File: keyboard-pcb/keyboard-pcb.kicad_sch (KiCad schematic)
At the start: 131 parts, among them SW1 RotaryEncoder_Switch, U1 Pico

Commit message: added footprints to pcb editor
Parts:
- U1: footprint RPi_Pico:RPi_Pico_SMD_TH -> MCU_RaspberryPi_and_Boards:RPi_Pico_SMD_TH
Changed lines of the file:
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@@
     (property "Reference" "U1" (id 0) (at 76.2 36.83 0))
     (property "Value" "Pico" (id 1) (at 76.2 39.37 0))
-    (property "Footprint" "RPi_Pico:RPi_Pico_SMD_TH" (id 2) (at 76.2 68.58 90)
+    (property "Footprint" "MCU_RaspberryPi_and_Boards:RPi_Pico_SMD_TH" (id 2) (at 76.2 68.58 90)
       (effects (font (size 1.27 1.27)) hide)
     )
@@
     )
     (path "/f433be38-82e2-473b-9bcf-c0c050d04e9a"
-      (reference "U1") (unit 1) (value "Pico") (footprint "RPi_Pico:RPi_Pico_SMD_TH")
+      (reference "U1") (unit 1) (value "Pico") (footprint "MCU_RaspberryPi_and_Boards:RPi_Pico_SMD_TH")
     )
     (path "/c4b08a63-44b5-48b9-adfd-68736c92ed66"

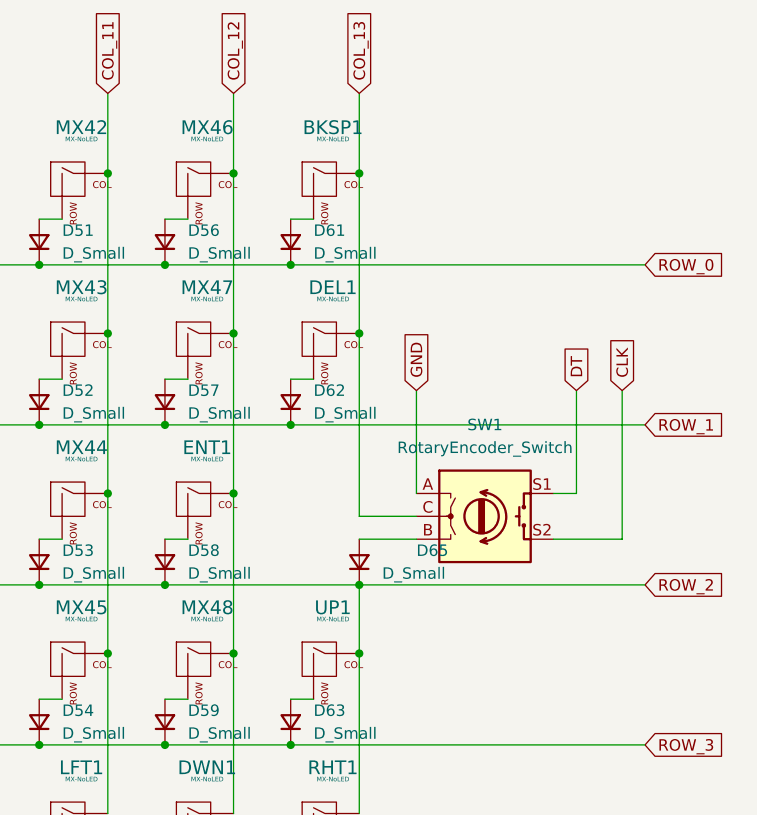
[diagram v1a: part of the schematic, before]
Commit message: fixed error in schematic and moved rotary encoder up
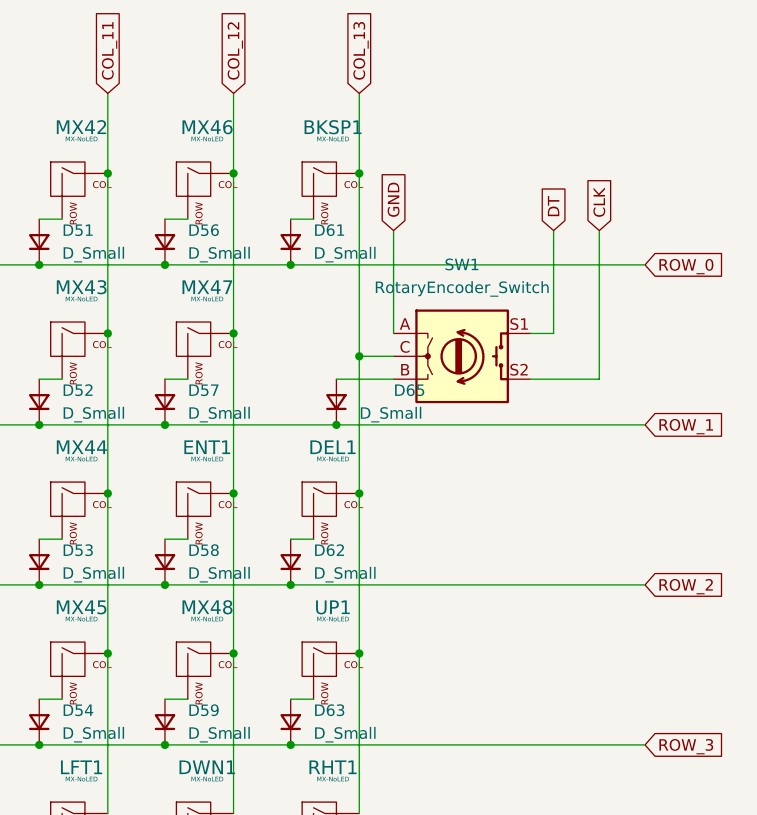
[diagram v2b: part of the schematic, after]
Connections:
- net COL_13: now also RHT1.1 (COL), UP1.1 (COL)
- net ROW_1: now also D65.1 (K); no longer D62.1 (K)
- net ROW_2: now also D62.1 (K); no longer D65.1 (K), RHT1.1 (COL), UP1.1 (COL)
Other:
- moved on the sheet: D62, D65, DEL1, SW1

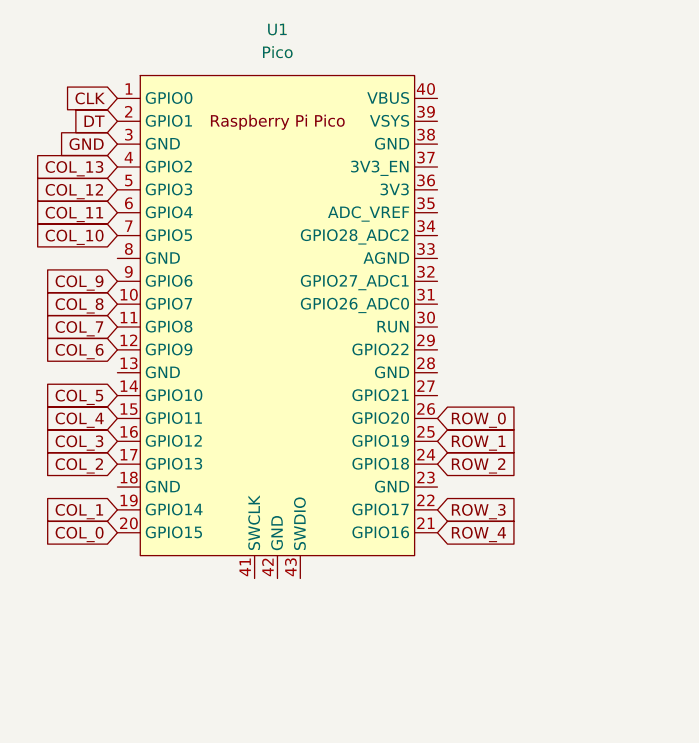
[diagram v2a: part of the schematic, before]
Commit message: routed key matric with tracks
+ rows and rotary encoder connected to GPIO pins
* still need to connect remaining columns
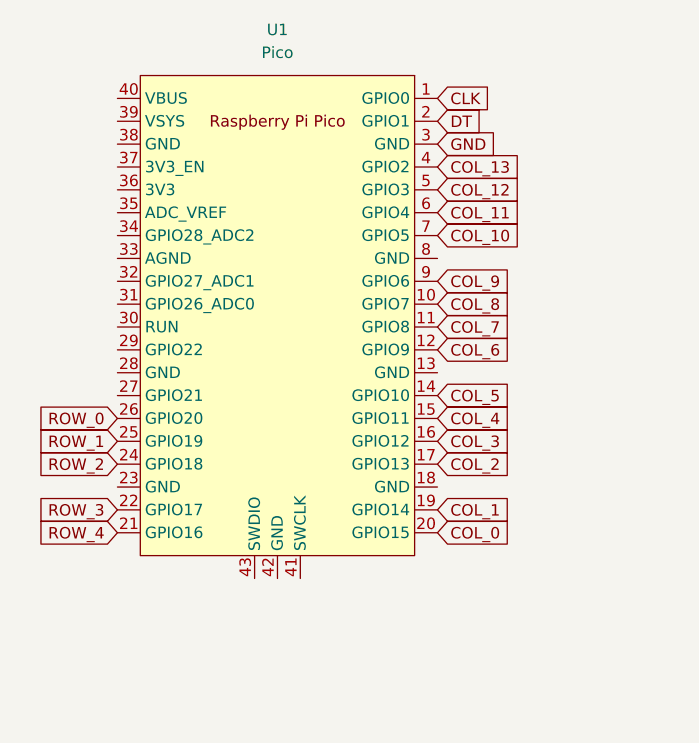
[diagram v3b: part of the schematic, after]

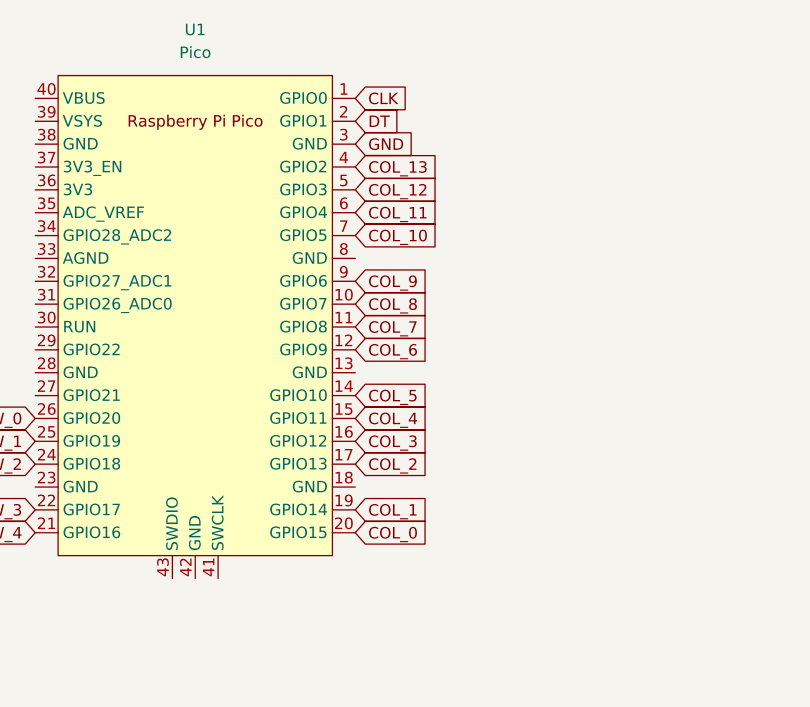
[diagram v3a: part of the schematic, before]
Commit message: added column GPIO tracks - pcb completed
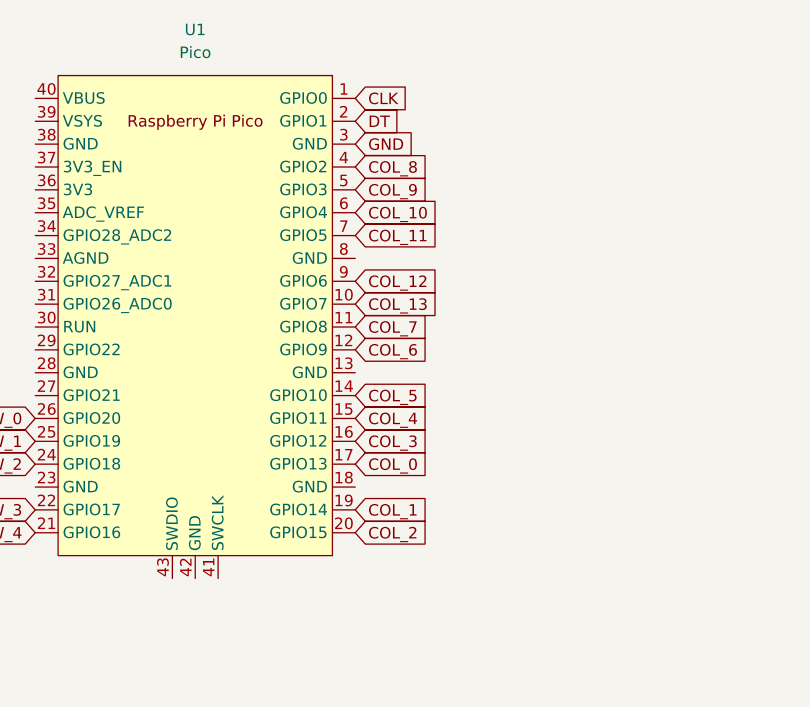
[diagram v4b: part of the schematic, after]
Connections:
- net COL_0: now also U1.17 (GPIO13); no longer U1.20 (GPIO15)
- net COL_10: now also U1.6 (GPIO4); no longer U1.7 (GPIO5)
- net COL_11: now also U1.7 (GPIO5); no longer U1.6 (GPIO4)
- net COL_12: now also U1.9 (GPIO6); no longer U1.5 (GPIO3)
- net COL_13: now also U1.10 (GPIO7); no longer U1.4 (GPIO2)
- net COL_2: now also U1.20 (GPIO15); no longer U1.17 (GPIO13)
- net COL_8: now also U1.4 (GPIO2); no longer U1.10 (GPIO7)
- net COL_9: now also U1.5 (GPIO3); no longer U1.9 (GPIO6)
